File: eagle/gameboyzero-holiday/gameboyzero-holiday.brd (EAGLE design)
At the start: 71 x 94 mm, 27 parts

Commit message: Wed 25 Oct 2017 09:07:01 EDT - holiday express board released
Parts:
- R1: value 100 -> 3R9
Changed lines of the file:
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@@
 </autorouter>
 <elements>
-<element name="R1" library="adafruit" library_urn="urn:adsk.eagle:library:420" package="R0805" value="100" x="2.6" y="36.5" smashed="yes" rot="R180"/>
+<element name="R1" library="adafruit" library_urn="urn:adsk.eagle:library:420" package="R0805" value="3R9" x="2.6" y="36.5" smashed="yes" rot="R180"/>
 <element name="PI1" library="RPI-Zero" package="RASPBERRYPI_BASTELSTUBE_V13_RASPI_BOARD_B+_FULL" value="RPI-ZERO" x="0.445" y="88.27" rot="MR180"/>
 <element name="SCREEN1" library="GameboyZeroHandheldDisplays" package="GAMEBOYZEROHANDHELDDISPLAYS-2.8" value="GAMEBOYZEROHANDHELDDISPLAYS-2.8" x="35.5" y="63" smashed="yes"/>

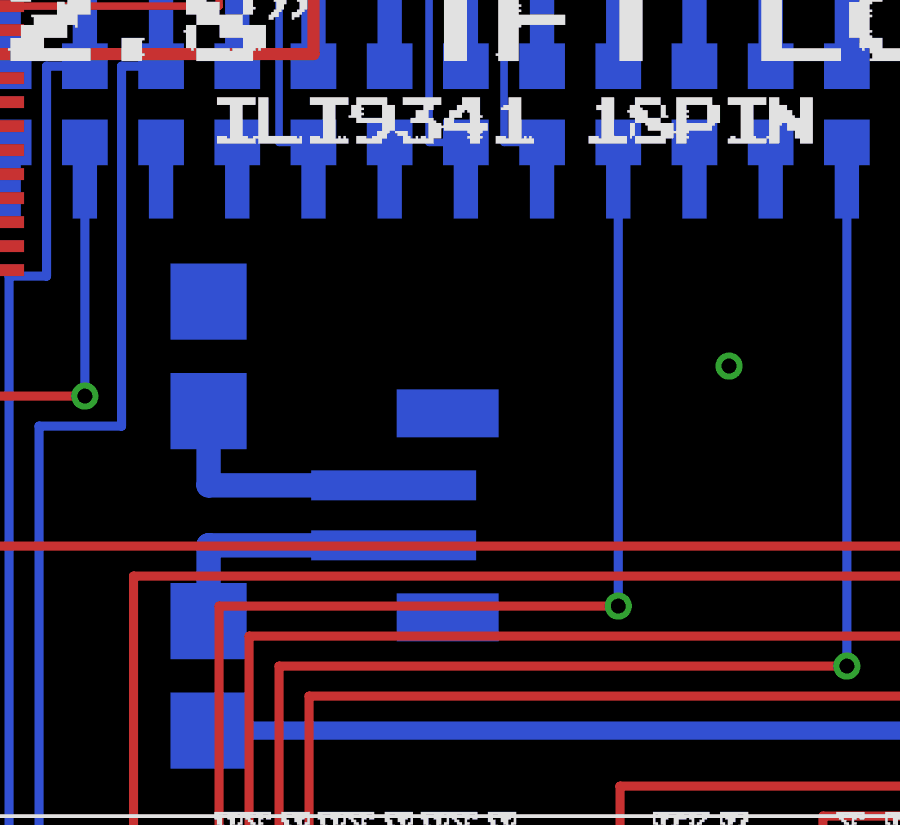
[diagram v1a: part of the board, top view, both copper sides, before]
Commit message: updates
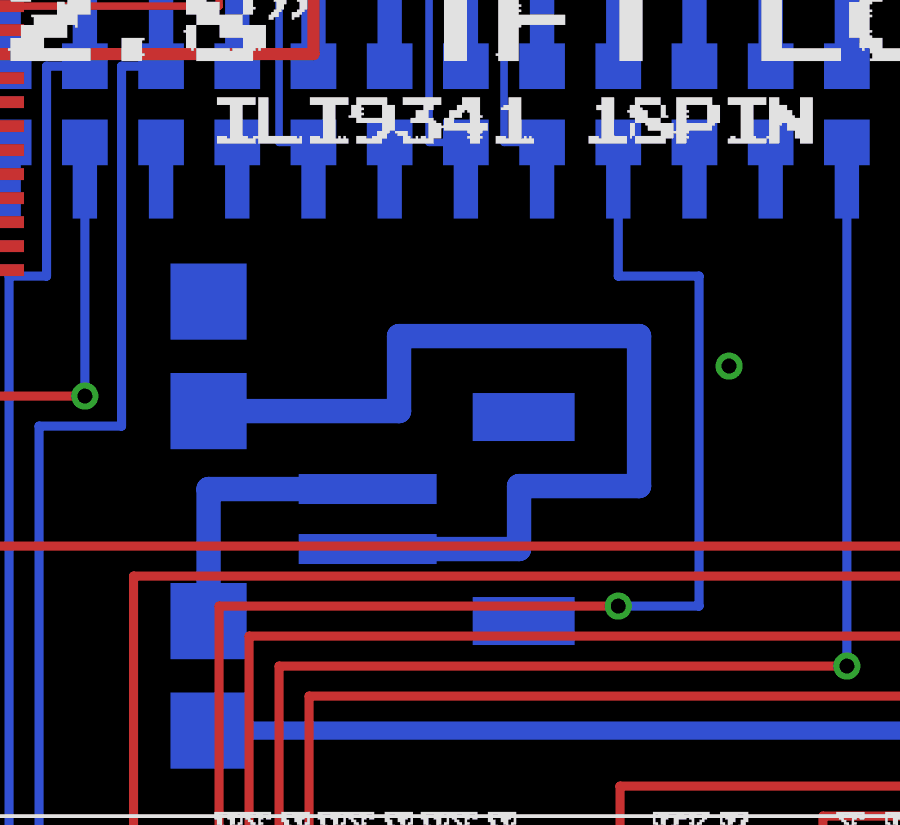
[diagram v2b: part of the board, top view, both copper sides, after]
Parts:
- removed CN1: (no value), adafruit:JST-PH-2-SMT
- added J1: (no value), SparkFun-Connectors:JST-2-SMD
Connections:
- net BATT+: now also J1.2; no longer CN1.1
- net BATT-: now also J1.1; no longer CN1.2
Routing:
- net BATT-: track 8.65 -> 33.0 mm
- net UP: track 55.8 -> 61.0 mm
- net BATT+: track 8.70 -> 9.71 mm
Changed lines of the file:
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@@
 <setting verticaltext="up"/>
 </settings>
-<grid distance="0.086" unitdist="mm" unit="mm" style="lines" multiple="1" display="yes" altdistance="0.25" altunitdist="mm" altunit="mm"/>
+<grid distance="1" unitdist="mm" unit="mm" style="lines" multiple="1" display="yes" altdistance="0.25" altunitdist="mm" altunit="mm"/>
 <layers>
 <layer number="1" name="Top" color="4" fill="1" visible="yes" active="yes"/>
-<layer number="2" name="Route2" color="1" fill="3" visible="yes" active="yes"/>
-<layer number="15" name="Route15" color="4" fill="6" visible="yes" active="yes"/>
+<layer number="2" name="Route2" color="1" fill="3" visible="no" active="yes"/>
+<layer number="15" name="Route15" color="4" fill="6" visible="no" active="yes"/>
 <layer number="16" name="Bottom" color="1" fill="1" visible="yes" active="yes"/>
 <layer number="17" name="Pads" color="2" fill="1" visible="yes" active="yes"/>
@@
 <element name="PI1" library="RPI-Zero" package="RASPBERRYPI_BASTELSTUBE_V13_RASPI_BOARD_B+_FULL" value="RPI-ZERO" x="0.445" y="88.27" rot="MR180"/>
 <element name="SCREEN1" library="GameboyZeroHandheldDisplays" package="GAMEBOYZEROHANDHELDDISPLAYS-2.8" value="GAMEBOYZEROHANDHELDDISPLAYS-2.8" x="35.5" y="63" smashed="yes"/>
-<element name="CN1" library="adafruit" library_urn="urn:adsk.eagle:library:420" package="JST-PH-2-SMT" value="" x="33.62" y="48.025" smashed="yes" rot="MR90">
-<attribute name="VALUE" x="26" y="45.485" size="1.27" layer="28" font="vector" rot="MR90"/>
-</element>
 <element name="POWER1" library="03962A" package="03962A" value="03962A" x="27" y="56.5" smashed="yes" rot="MR270"/>
 <element name="BTN_X" library="SparkFun-Switches" library_urn="urn:adsk.eagle:library:535" package="TACTILE_SWITCH_SMD_12MM" package3d_urn="urn:adsk.eagle:package:40166/1" value="MOMENTARY-SWITCH-SPST-SMD-12MM" x="53.82985" y="28.2782" smashed="yes" rot="R70">
@@
 <element name="H4" library="holes" library_urn="urn:adsk.eagle:library:237" package="2,8" package3d_urn="urn:adsk.eagle:package:14271/1" value="MOUNT-HOLE2.8" x="4" y="91"/>
 <element name="H5" library="holes" library_urn="urn:adsk.eagle:library:237" package="2,8" package3d_urn="urn:adsk.eagle:package:14271/1" value="MOUNT-HOLE2.8" x="67" y="91"/>
+<element name="J1" library="SparkFun-Connectors" package="JST-2-SMD" value="" x="34.654" y="47.902" rot="MR90">
+<attribute name="BTM_NEG" value="-" x="34.654" y="47.902" size="1.778" layer="28" rot="MR90" display="off"/>
+<attribute name="BTM_POS" value="+" x="34.654" y="47.902" size="1.778" layer="28" rot="MR90" display="off"/>
+<attribute name="PROD_ID" value="CONN-11443" x="34.654" y="47.902" size="1.778" layer="28" rot="MR90" display="off"/>
+<attribute name="TOP_NEG" value="-" x="34.654" y="47.902" size="1.778" layer="28" rot="MR90" display="off"/>
+<attribute name="TOP_POS" value="+" x="34.654" y="47.902" size="1.778" layer="28" rot="MR90" display="off"/>
+</element>
 </elements>
 <signals>
@@
 <contactref element="PI1" pad="26"/>
 <contactref element="BTN_UP" pad="B2"/>
-<wire x1="39.307" y1="59" x2="39.307" y2="45" width="0.3048" layer="16"/>
 <wire x1="16.21975625" y1="27.9017375" x2="26" y2="27.9017375" width="0.3048" layer="1"/>
 <wire x1="26" y1="27.9017375" x2="26" y2="45" width="0.3048" layer="1"/>
@@
 <contactref element="PI1" pad="66"/>
 <wire x1="39.307" y1="60.457" x2="39.307" y2="59" width="0.254" layer="16"/>
-<wire x1="39.307" y1="58.806" x2="39.307" y2="59" width="0.4064" layer="16"/>
+<wire x1="39.307" y1="59" x2="39.307" y2="58.806" width="0.4064" layer="16"/>
+<wire x1="39.307" y1="58.806" x2="39.307" y2="56" width="0.3048" layer="16"/>
+<wire x1="39.307" y1="56" x2="42" y2="56" width="0.3048" layer="16"/>
+<wire x1="42" y1="56" x2="42" y2="45" width="0.3048" layer="16"/>
+<wire x1="42" y1="45" x2="39.307" y2="45" width="0.3048" layer="16"/>
 </signal>
 <signal name="SWITCH_OUT+">
@@
 <signal name="BATT+">
 <contactref element="POWER1" pad="B+"/>
-<contactref element="CN1" pad="1"/>
-<wire x1="31.82" y1="47.025" x2="25.65" y2="47.025" width="0.8128" layer="16"/>
-<wire x1="25.65" y1="47.025" x2="25.65" y2="44.5" width="0.8128" layer="16"/>
+<contactref element="J1" pad="2"/>
+<wire x1="25.65" y1="44.5" x2="25.65" y2="48.902" width="0.8128" layer="16"/>
+<wire x1="25.65" y1="48.902" x2="30.954" y2="48.902" width="0.8128" layer="16"/>
 </signal>
 <signal name="BATT-">
 <contactref element="POWER1" pad="B-"/>
-<wire x1="25.65" y1="49.025" x2="25.65" y2="51.5" width="0.8128" layer="16"/>
-<contactref element="CN1" pad="2"/>
-<wire x1="31.82" y1="49.025" x2="25.65" y2="49.025" width="0.8128" layer="16"/>
+<contactref element="J1" pad="1"/>
+<wire x1="25.65" y1="51.5" x2="32" y2="51.5" width="0.8128" layer="16"/>
+<wire x1="32" y1="51.5" x2="32" y2="54" width="0.8128" layer="16"/>
+<wire x1="32" y1="54" x2="40" y2="54" width="0.8128" layer="16"/>
+<wire x1="40" y1="54" x2="40" y2="49" width="0.8128" layer="16"/>
+<wire x1="40" y1="49" x2="36" y2="49" width="0.8128" layer="16"/>
+<wire x1="36" y1="46.902" x2="30.954" y2="46.902" width="0.8128" layer="16"/>
+<wire x1="36" y1="49" x2="36" y2="46.902" width="0.8128" layer="16"/>
 </signal>
 <signal name="SWITCH_IN+">
